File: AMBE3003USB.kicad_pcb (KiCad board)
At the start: 2 copper layers, 95 x 85 mm, 208 parts, among them J1 McBSP, J2 USB_OTG, J4 CODEC, P1 GND, P2 Config, P3 3v3, P4 VSET, P5 HARD RESET, P6 SEQ, P7 3v3, P8 ACONF, P9 GND, Q1 BC847, U1 AMBE3003, U2 TPS75005RGW_wPin21, U3 FT232RL, X1 29.4912

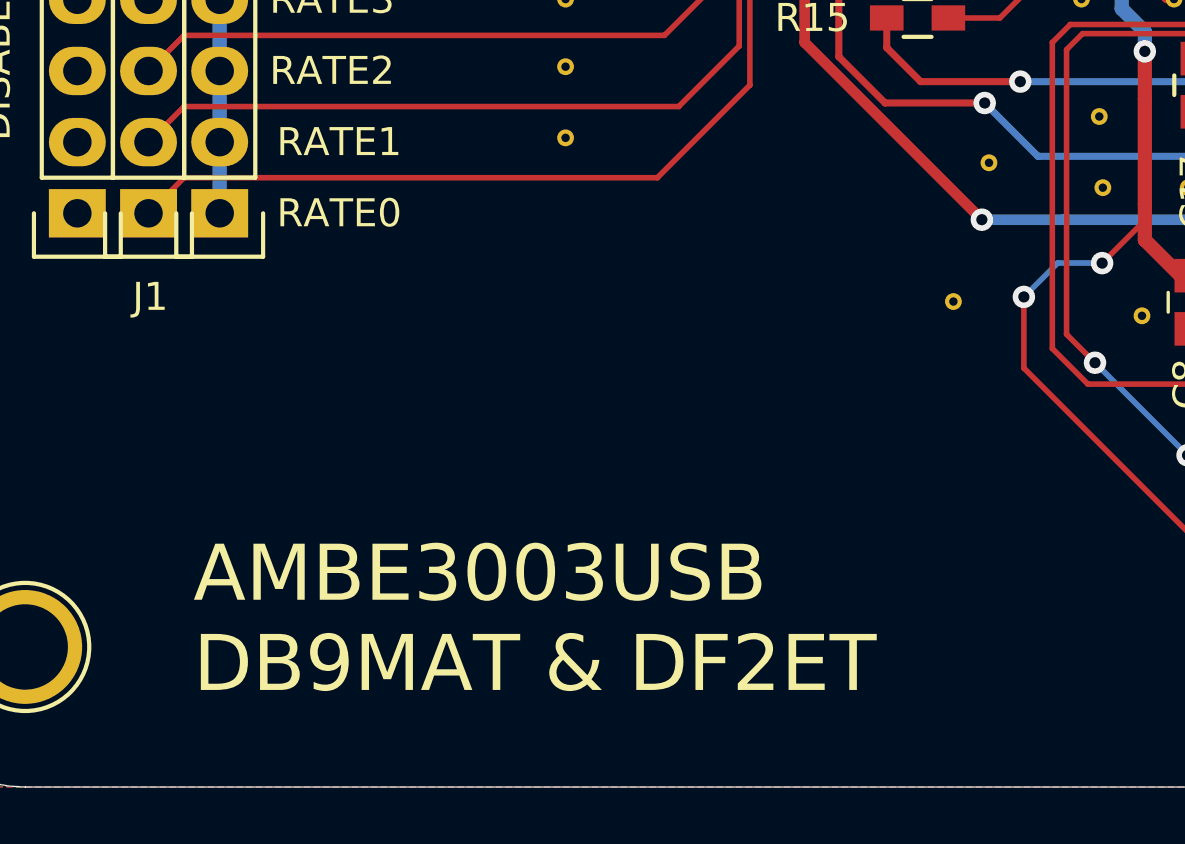
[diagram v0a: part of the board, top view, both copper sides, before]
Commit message: Add nice logo
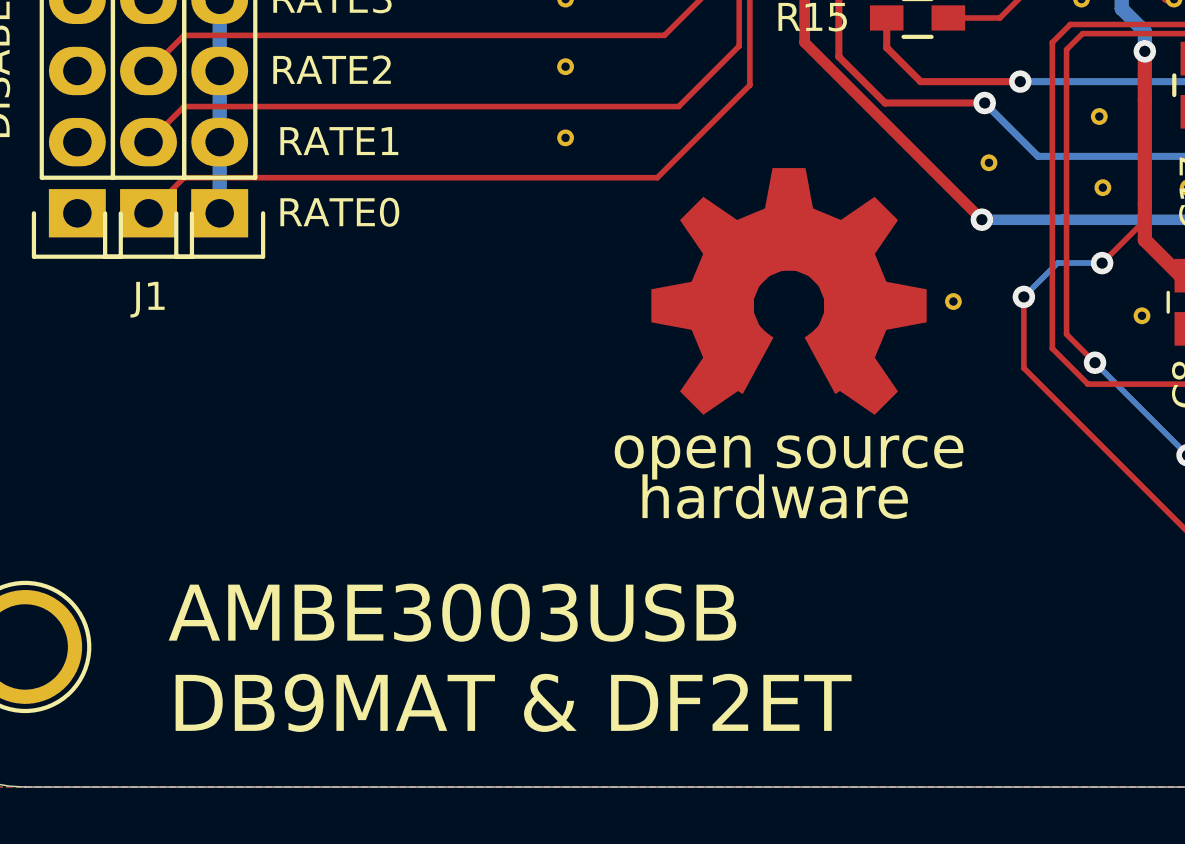
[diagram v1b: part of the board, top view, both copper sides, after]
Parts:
- added OSHW_COPPER_10MM: VAL**, Symbols:OSHW_COPPER_10MM, F.Cu at (64.3, 115.8)
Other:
- board text added: "hardware"
- board text added: "open source"
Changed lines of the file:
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@@
     (links 392)
     (no_connects 0)
-    (area 31.974499 47.974499 127.025501 133.025501)
+    (area 31.974499 41.5 138.65 133.025501)
     (thickness 1.6)
-    (drawings 159)
+    (drawings 161)
     (tracks 1325)
     (zones 0)
-    (modules 208)
+    (modules 209)
     (nets 85)
   )
@@
       (drillshape 0)
       (scaleselection 1)
-      (outputdirectory /opt/AMBE3003USB/))
+      (outputdirectory /opt/AMBE3003USB/gerbers/))
   )
   (net 0 "")
@@
     )
   )
+  (module Symbols:OSHW_COPPER_10MM (layer F.Cu)
+    (at 64.262 115.824)
+    (fp_text reference OSHW_COPPER_10MM (at 0 5.461) (layer F.SilkS) hide
+      (effects (font (thickness 0.3048)))
+    )
+    (fp_text value VAL** (at 0 -7.239) (layer F.SilkS) hide
+      (effects (font (thickness 0.3048)))
+    )
+    (pad "" smd trapezoid (at 0 -4.1656 180) (size 1.45796 1.4986) (rect_delta 0 -0.2794 ) (layers F.Cu F.Paste F.Mask))
+    (pad "" smd trapezoid (at 2.94386 -2.94386 135) (size 1.45796 1.4986) (rect_delta 0 -0.2794 ) (layers F.Cu F.Paste F.Mask))
+    (pad "" smd trapezoid (at 4.1656 0 90) (size 1.45796 1.4986) (rect_delta 0 -0.2794 ) (layers F.Cu F.Paste F.Mask))
+    (pad "" smd trapezoid (at 2.94386 2.94386 45) (size 1.45796 1.4986) (rect_delta 0 -0.2794 ) (layers F.Cu F.Paste F.Mask))
+    (pad "" smd trapezoid (at -2.94386 -2.94386 225) (size 1.45796 1.4986) (rect_delta 0 -0.2794 ) (layers F.Cu F.Paste F.Mask))
+    (pad "" smd trapezoid (at -4.1656 0 270) (size 1.45796 1.4986) (rect_delta 0 -0.2794 ) (layers F.Cu F.Paste F.Mask))
+    (pad "" smd trapezoid (at -2.94386 2.94386 315) (size 1.45796 1.4986) (rect_delta 0 -0.2794 ) (layers F.Cu F.Paste F.Mask))
+    (pad "" smd trapezoid (at 0 -2.39522 180) (size 1.08204 2.29108) (rect_delta 0 0.41402 ) (layers F.Cu F.Paste F.Mask))
+    (pad "" smd trapezoid (at -0.9144 -2.21234 202.5) (size 1.08204 2.29108) (rect_delta 0 0.41402 ) (layers F.Cu F.Paste F.Mask))
+    (pad "" smd trapezoid (at 0.9144 -2.21234 157.5) (size 1.08204 2.29108) (rect_delta 0 0.41402 ) (layers F.Cu F.Paste F.Mask))
+    (pad "" smd trapezoid (at 1.69164 -1.69164 135) (size 1.08204 2.29108) (rect_delta 0 0.41402 ) (layers F.Cu F.Paste F.Mask))
+    (pad "" smd trapezoid (at -1.69164 -1.69164 225) (size 1.08204 2.29108) (rect_delta 0 0.41402 ) (layers F.Cu F.Paste F.Mask))
+    (pad "" smd trapezoid (at 2.21234 -0.9144 112.5) (size 1.08204 2.29108) (rect_delta 0 0.41402 ) (layers F.Cu F.Paste F.Mask))
+    (pad "" smd trapezoid (at -2.21234 -0.9144 247.5) (size 1.08204 2.29108) (rect_delta 0 0.41402 ) (layers F.Cu F.Paste F.Mask))
+    (pad "" smd trapezoid (at 2.39522 0 90) (size 1.08204 2.29108) (rect_delta 0 0.41402 ) (layers F.Cu F.Paste F.Mask))
+    (pad "" smd trapezoid (at -2.39522 0 270) (size 1.08204 2.29108) (rect_delta 0 0.41402 ) (layers F.Cu F.Paste F.Mask))
+    (pad "" smd trapezoid (at -2.21234 0.9144 292.5) (size 1.08204 2.29108) (rect_delta 0 0.41402 ) (layers F.Cu F.Paste F.Mask))
+    (pad "" smd trapezoid (at 2.21234 0.9144 67.5) (size 1.08204 2.29108) (rect_delta 0 0.41402 ) (layers F.Cu F.Paste F.Mask))
+    (pad "" smd trapezoid (at 1.69164 1.69164 45) (size 1.08204 2.29108) (rect_delta 0 0.41402 ) (layers F.Cu F.Paste F.Mask))
+    (pad "" smd trapezoid (at -1.69164 1.69164 315) (size 1.08204 2.29108) (rect_delta 0 0.41402 ) (layers F.Cu F.Paste F.Mask))
+    (pad "" smd trapezoid (at -1.32842 1.99136 326.3) (size 0.54102 2.29108) (rect_delta 0 0.20828 ) (layers F.Cu F.Paste F.Mask))
+    (pad "" smd trapezoid (at 1.32842 1.99136 33.7) (size 0.54102 2.29108) (rect_delta 0 0.20828 ) (layers F.Cu F.Paste F.Mask))
+  )
+  (gr_text hardware (at 63.7286 122.7074) (layer F.SilkS)
+    (effects (font (size 1.5 1.5) (thickness 0.3)))
+  )
+  (gr_text "open source" (at 64.262 120.904) (layer F.SilkS)
+    (effects (font (size 1.5 1.5) (thickness 0.3)))
+  )
   (gr_text P2 (at 115.8875 112.141) (layer F.SilkS)
     (effects (font (size 1 1) (thickness 0.15)))
@@
     (effects (font (size 1 1) (thickness 0.15)))
   )
-  (gr_text "AMBE3003USB\nDB9MAT & DF2ET" (at 43 127) (layer F.SilkS)
+  (gr_text "AMBE3003USB\nDB9MAT & DF2ET" (at 42.1005 128.4605) (layer F.SilkS)
     (effects (font (size 2 2) (thickness 0.5)) (justify left))
   )
